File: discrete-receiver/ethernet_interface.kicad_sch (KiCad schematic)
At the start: 16 parts, among them J6 SI-52003-F, U9 LAN8720A

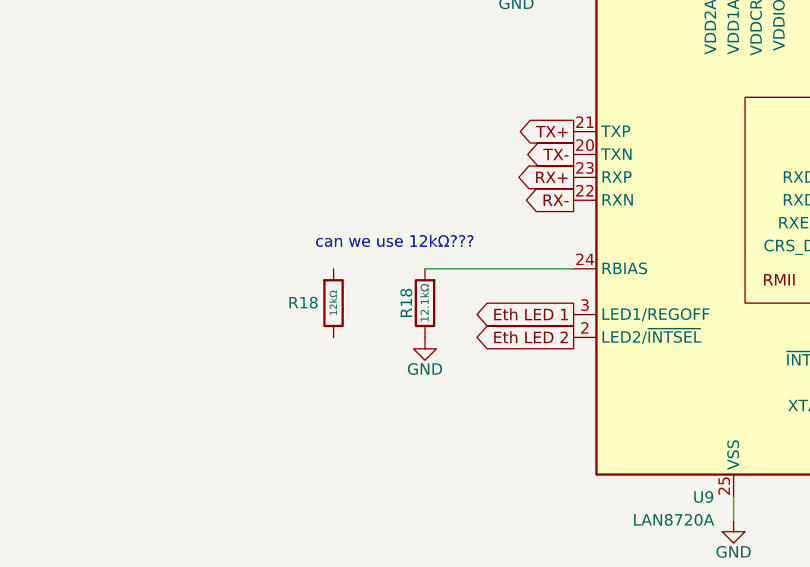
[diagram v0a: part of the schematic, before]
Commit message: Updated schematic
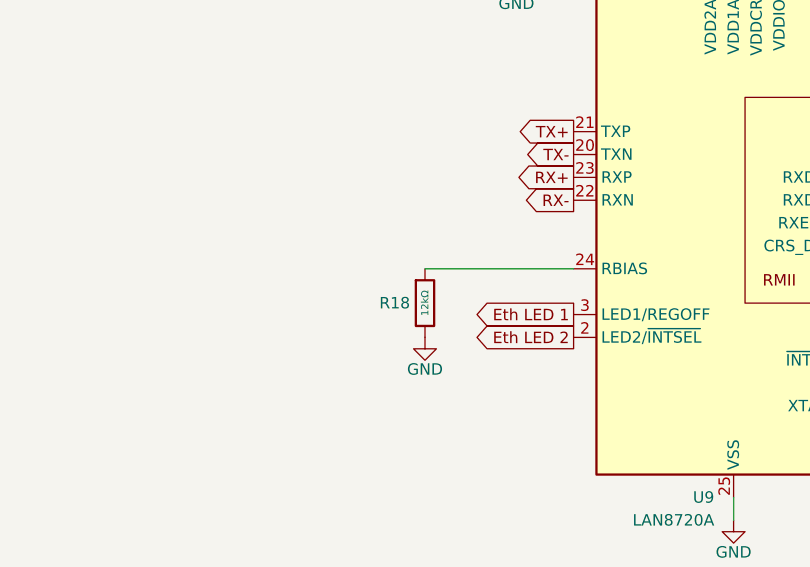
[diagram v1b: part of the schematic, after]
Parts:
- removed R18: 12.1kΩ, symbol Device:R
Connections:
- net GND: now also R18.2
- net at U9.24 (RBIAS): now also R18.1
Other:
- note removed: "can we use 12kΩ???"
- moved on the sheet: R18
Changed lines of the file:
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@@
 	(generator_version "10.0")
 	(paper "A4")
-	(text "can we use 12kΩ???"
-		(exclude_from_sim no)
-		(at 152.908 93.726 0)
-		(effects
-			(font
-				(size 1.27 1.27)
-			)
-			(justify left)
-		)
-	)
 	(text "These LEDs are wired such that nINTSEL is pulled low.\nThis causes the LAN8720a to drive the LEDs active high.\nWe've also ensured that REGOFF is set to zero such that\nthe internal 1.2V regulator is enabled."
 		(exclude_from_sim no)
@@
 	(symbol
 		(lib_id "PCM_JLCPCB-Resistors:0402,12kΩ")
-		(at 154.94 100.33 0)
+		(at 165.1 100.33 0)
 		(unit 1)
 		(body_style 1)
@@
 		(dnp no)
 		(property "Reference" "R18"
-			(at 149.86 100.33 0)
+			(at 160.02 100.33 0)
 			(show_name no)
 			(do_not_autoplace no)
@@
 		)
 		(property "Value" "12kΩ"
-			(at 154.94 100.33 90)
+			(at 165.1 100.33 90)
 			(show_name no)
 			(do_not_autoplace yes)
@@
 		)
 		(property "Footprint" "PCM_JLCPCB:R_0402"
-			(at 153.162 100.33 90)
+			(at 163.322 100.33 90)
 			(hide yes)
 			(show_name no)
@@
 		)
 		(property "Datasheet" "https://www.lcsc.com/datasheet/lcsc_datasheet_2206010100_UNI-ROYAL-Uniroyal-Elec-0402WGF1202TCE_C25752.pdf"
-			(at 154.94 100.33 0)
+			(at 165.1 100.33 0)
 			(hide yes)
 			(show_name no)
@@
 		)
 		(property "Description" "62.5mW Thick Film Resistors 50V ±100ppm/°C ±1% 12kΩ 0402 Chip Resistor - Surface Mount ROHS"
-			(at 154.94 100.33 0)
+			(at 165.1 100.33 0)
 			(hide yes)
 			(show_name no)
@@
 		)
 		(property "LCSC" "C25752"
-			(at 154.94 100.33 0)
+			(at 165.1 100.33 0)
 			(hide yes)
 			(show_name no)
@@
 		)
 		(property "Stock" "342039"
-			(at 154.94 100.33 0)
+			(at 165.1 100.33 0)
 			(hide yes)
 			(show_name no)
@@
 		)
 		(property "Price" "0.004USD"
-			(at 154.94 100.33 0)
+			(at 165.1 100.33 0)
 			(hide yes)
 			(show_name no)
@@
 		)
 		(property "Process" "SMT"
-			(at 154.94 100.33 0)
+			(at 165.1 100.33 0)
 			(hide yes)
 			(show_name no)
@@
 		)
 		(property "Minimum Qty" "20"
-			(at 154.94 100.33 0)
+			(at 165.1 100.33 0)
 			(hide yes)
 			(show_name no)
@@
 		)
 		(property "Attrition Qty" "10"
-			(at 154.94 100.33 0)
+			(at 165.1 100.33 0)
 			(hide yes)
 			(show_name no)
@@
 		)
 		(property "Class" "Basic Component"
-			(at 154.94 100.33 0)
+			(at 165.1 100.33 0)
 			(hide yes)
 			(show_name no)
@@
 		)
 		(property "Category" "Resistors,Chip Resistor - Surface Mount"
-			(at 154.94 100.33 0)
+			(at 165.1 100.33 0)
 			(hide yes)
 			(show_name no)
@@
 		)
 		(property "Manufacturer" "UNI-ROYAL(Uniroyal Elec)"
-			(at 154.94 100.33 0)
+			(at 165.1 100.33 0)
 			(hide yes)
 			(show_name no)
@@
 		)
 		(property "Part" "0402WGF1202TCE"
-			(at 154.94 100.33 0)
+			(at 165.1 100.33 0)
 			(hide yes)
 			(show_name no)
@@
 		)
 		(property "Resistance" "12kΩ"
-			(at 154.94 100.33 0)
+			(at 165.1 100.33 0)
 			(hide yes)
 			(show_name no)
@@
 		)
 		(property "Power(Watts)" "62.5mW"
-			(at 154.94 100.33 0)
+			(at 165.1 100.33 0)
 			(hide yes)
 			(show_name no)
@@
 		)
 		(property "Type" "Thick Film Resistors"
-			(at 154.94 100.33 0)
+			(at 165.1 100.33 0)
 			(hide yes)
 			(show_name no)
@@
 		)
 		(property "Overload Voltage (Max)" "50V"
-			(at 154.94 100.33 0)
+			(at 165.1 100.33 0)
 			(hide yes)
 			(show_name no)
@@
 		)
 		(property "Operating Temperature Range" "-55°C~+155°C"
-			(at 154.94 100.33 0)
+			(at 165.1 100.33 0)
 			(hide yes)
 			(show_name no)
@@
 		)
 		(property "Tolerance" "±1%"
-			(at 154.94 100.33 0)
+			(at 165.1 100.33 0)
 			(hide yes)
 			(show_name no)
@@
 		)
 		(property "Temperature Coefficient" "±100ppm/°C"
-			(at 154.94 100.33 0)
-			(hide yes)
-			(show_name no)
-			(do_not_autoplace no)
-			(effects
-				(font
-					(size 1.27 1.27)
-				)
-			)
-		)
-		(pin "2"
-		)
-		(pin "1"
-		)
-		(instances
-			(project "diode_tayloe_sdr"
-				(path "/d18d178d-3f10-4d68-9036-eae71a7d091a/09065ae7-5d3e-4f86-b983-86dca844c240"
-					(reference "R18")
-					(unit 1)
-				)
-			)
-		)
-	)
-	(symbol
-		(lib_id "Device:R")
-		(at 165.1 100.33 180)
-		(unit 1)
-		(body_style 1)
-		(exclude_from_sim no)
-		(in_bom yes)
-		(on_board yes)
-		(in_pos_files yes)
-		(dnp no)
-		(property "Reference" "R18"
-			(at 163.068 100.33 90)
-			(show_name no)
-			(do_not_autoplace no)
-			(effects
-				(font
-					(size 1.27 1.27)
-				)
-			)
-		)
-		(property "Value" "12.1kΩ"
-			(at 165.1 100.33 90)
-			(show_name no)
-			(do_not_autoplace no)
-			(effects
-				(font
-					(size 0.889 0.889)
-				)
-			)
-		)
-		(property "Footprint" ""
-			(at 166.878 100.33 90)
-			(hide yes)
-			(show_name no)
-			(do_not_autoplace no)
-			(effects
-				(font
-					(size 1.27 1.27)
-				)
-			)
-		)
-		(property "Datasheet" ""
 			(at 165.1 100.33 0)
 			(hide yes)
@@
 			)
 		)
-		(property "Description" "Resistor"
-			(at 165.1 100.33 0)
-			(hide yes)
-			(show_name no)
-			(do_not_autoplace no)
-			(effects
-				(font
-					(size 1.27 1.27)
-				)
-			)
+		(pin "2"
 		)
 		(pin "1"
 		)
-		(pin "2"
-		)
 		(instances
